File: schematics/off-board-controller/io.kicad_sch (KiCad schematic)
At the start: 44 parts, among them SW5 SW_SPDT_MSM, U8 MCP23S17_SP, U9 MCP23S17_SP

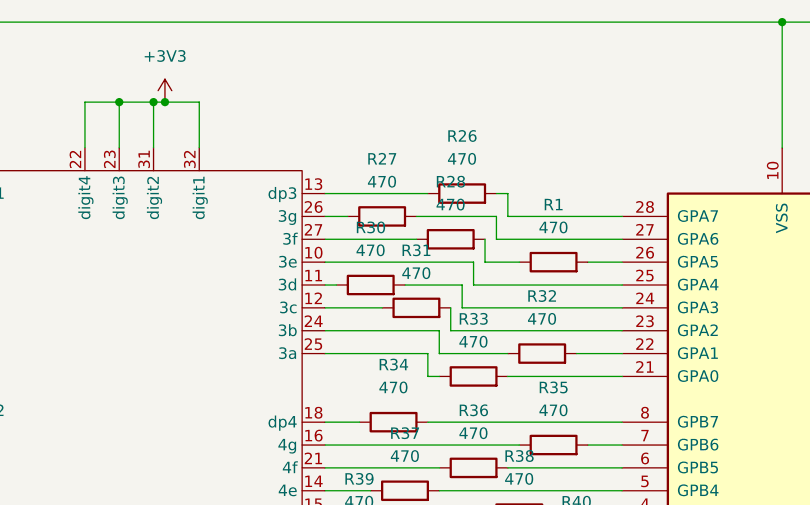
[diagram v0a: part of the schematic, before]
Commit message: layout
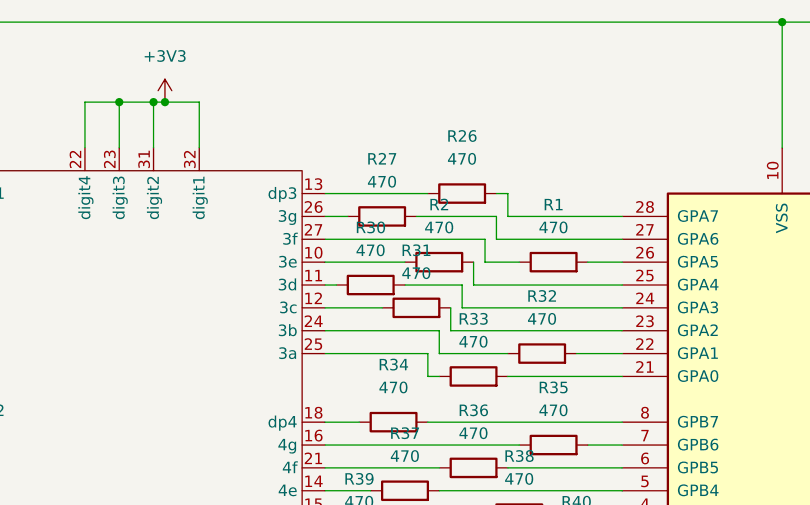
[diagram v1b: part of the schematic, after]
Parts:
- removed R28: 470, Resistor_SMD:R_0805_2012Metric_Pad1.20x1.40mm_HandSolder, symbol Device:R
- added R2: 470, Resistor_SMD:R_0805_2012Metric_Pad1.20x1.40mm_HandSolder, symbol Device:R
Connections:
- net at U10.10 (3e): now also R2.1; no longer U9.25 (GPA4)
- net at U10.27 (3f): now also R1.1
- new net: R2.2, U9.25 (GPA4)
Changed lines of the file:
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@@
 	(wire
 		(pts
-			(xy 147.32 45.72) (xy 137.16 45.72)
+			(xy 137.16 45.72) (xy 154.94 45.72)
 		)
 		(stroke
@@
 	(wire
 		(pts
-			(xy 137.16 48.26) (xy 153.67 48.26)
+			(xy 137.16 48.26) (xy 146.05 48.26)
 		)
 		(stroke
@@
 	(symbol
 		(lib_id "Device:R")
+		(at 149.86 48.26 90)
+		(unit 1)
+		(exclude_from_sim no)
+		(in_bom yes)
+		(on_board yes)
+		(dnp no)
+		(fields_autoplaced yes)
+		(property "Reference" "R2"
+			(at 149.86 41.91 90)
+			(effects
+				(font
+					(size 1.27 1.27)
+				)
+			)
+		)
+		(property "Value" "470"
+			(at 149.86 44.45 90)
+			(effects
+				(font
+					(size 1.27 1.27)
+				)
+			)
+		)
+		(property "Footprint" "Resistor_SMD:R_0805_2012Metric_Pad1.20x1.40mm_HandSolder"
+			(at 149.86 50.038 90)
+			(effects
+				(font
+					(size 1.27 1.27)
+				)
+				(hide yes)
+			)
+		)
+		(property "Datasheet" "~"
+			(at 149.86 48.26 0)
+			(effects
+				(font
+					(size 1.27 1.27)
+				)
+				(hide yes)
+			)
+		)
+		(property "Description" "Resistor"
+			(at 149.86 48.26 0)
+			(effects
+				(font
+					(size 1.27 1.27)
+				)
+				(hide yes)
+			)
+		)
+		(pin "2"
+		)
+		(pin "1"
+		)
+		(instances
+			(project "controller"
+				(path "/0775f04a-8a0e-41f5-b442-dacb2efdb863/92c85f3a-14b3-4661-ad21-779315976c0e"
+					(reference "R2")
+					(unit 1)
+				)
+			)
+		)
+	)
+	(symbol
+		(lib_id "Device:R")
 		(at 144.78 66.04 90)
 		(unit 1)
@@
 					(unit 1)
 				)
-			)
-		)
-	)
-	(symbol
-		(lib_id "Device:R")
-		(at 151.13 45.72 90)
-		(unit 1)
-		(exclude_from_sim no)
-		(in_bom yes)
-		(on_board yes)
-		(dnp no)
-		(fields_autoplaced yes)
-		(property "Reference" "R28"
-			(at 151.13 39.37 90)
-			(effects
-				(font
-					(size 1.27 1.27)
-				)
-			)
-		)
-		(property "Value" "470"
-			(at 151.13 41.91 90)
-			(effects
-				(font
-					(size 1.27 1.27)
-				)
-			)
-		)
-		(property "Footprint" "Resistor_SMD:R_0805_2012Metric_Pad1.20x1.40mm_HandSolder"
-			(at 151.13 47.498 90)
-			(effects
-				(font
-					(size 1.27 1.27)
-				)
-				(hide yes)
-			)
-		)
-		(property "Datasheet" "~"
-			(at 151.13 45.72 0)
-			(effects
-				(font
-					(size 1.27 1.27)
-				)
-				(hide yes)
-			)
-		)
-		(property "Description" "Resistor"
-			(at 151.13 45.72 0)
-			(effects
-				(font
-					(size 1.27 1.27)
-				)
-				(hide yes)
-			)
-		)
-		(pin "2"
-		)
-		(pin "1"
-		)
-		(instances
-			(project "controller"
-				(path "/0775f04a-8a0e-41f5-b442-dacb2efdb863/92c85f3a-14b3-4661-ad21-779315976c0e"
-					(reference "R28")
-					(unit 1)
-				)
